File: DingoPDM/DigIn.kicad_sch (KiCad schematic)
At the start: 6 parts

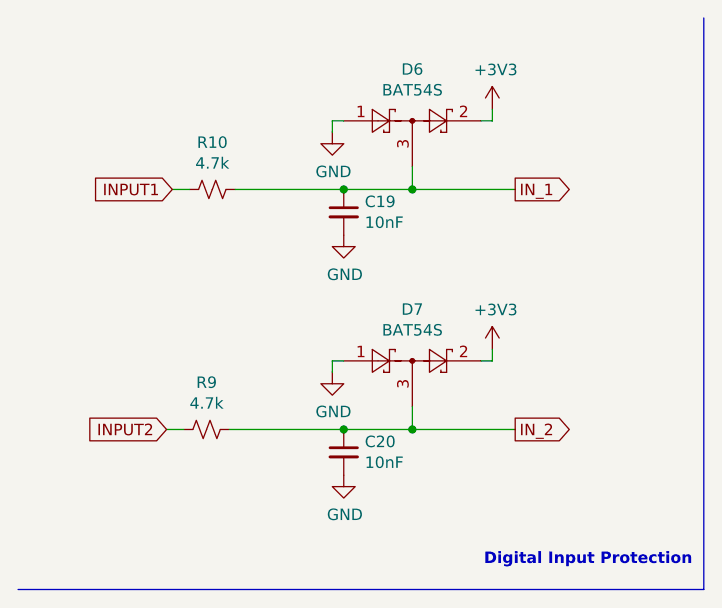
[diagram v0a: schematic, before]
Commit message: Routed V7
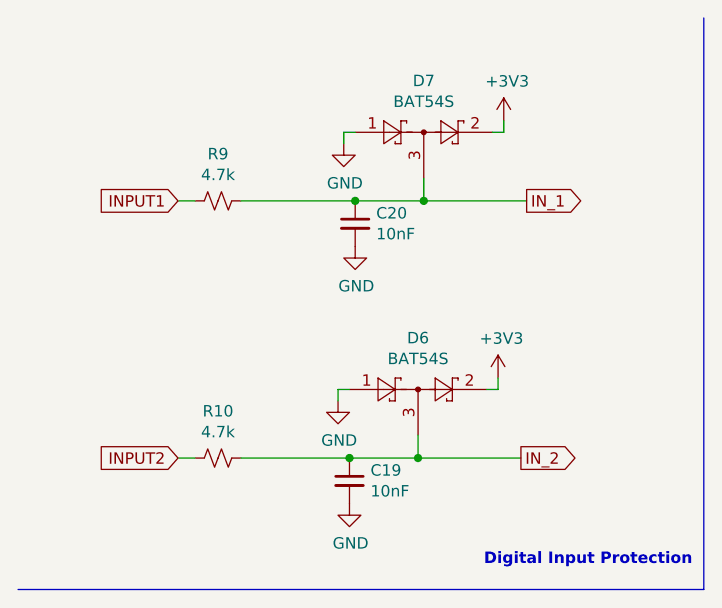
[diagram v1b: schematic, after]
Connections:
- net INPUT1: now also R9.2; no longer R10.2
- net INPUT2: now also R10.2; no longer R9.2
- net IN_1: now also C20.1, D7.3, R9.1; no longer C19.1, D6.3, R10.1
- net IN_2: now also C19.1, D6.3, R10.1; no longer C20.1, D7.3, R9.1
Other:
- moved on the sheet: C19, C20, D6, D7, R10, R9
